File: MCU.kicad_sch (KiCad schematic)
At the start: 32 parts, among them J4 2125281600, J5 Conn_02x08_Odd_Even, J6 Conn_02x08_Odd_Even, U7 STM32F405RGTx, Y1 8MHz

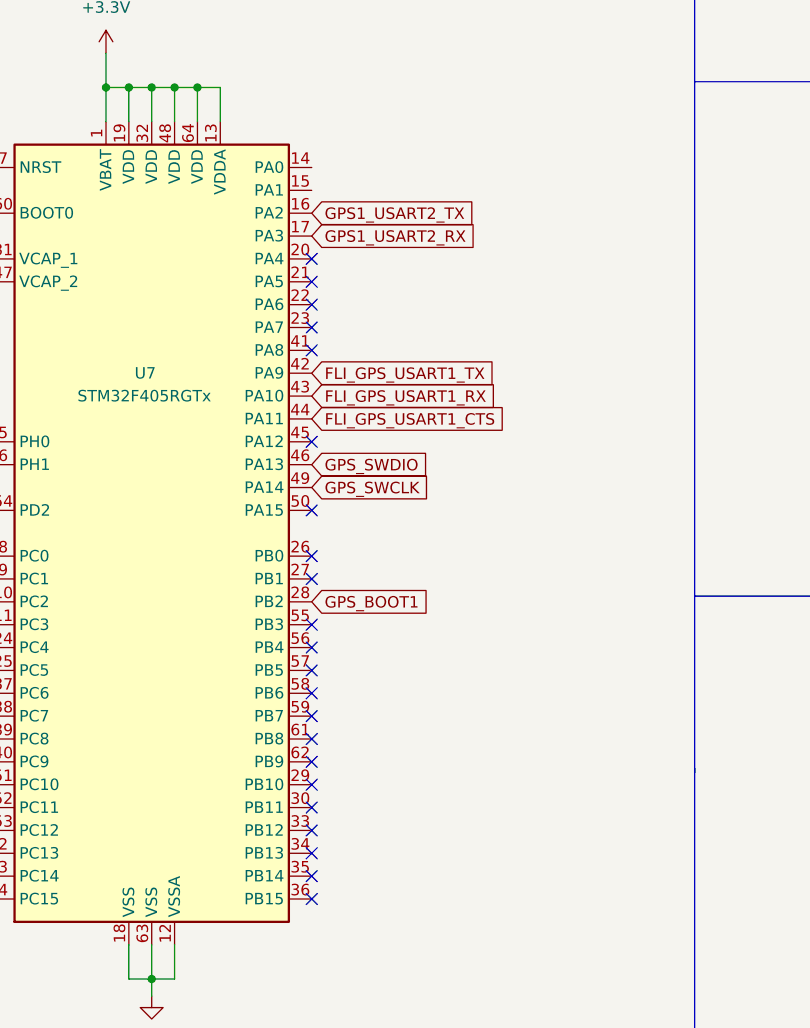
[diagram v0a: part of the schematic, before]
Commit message: Finished M10
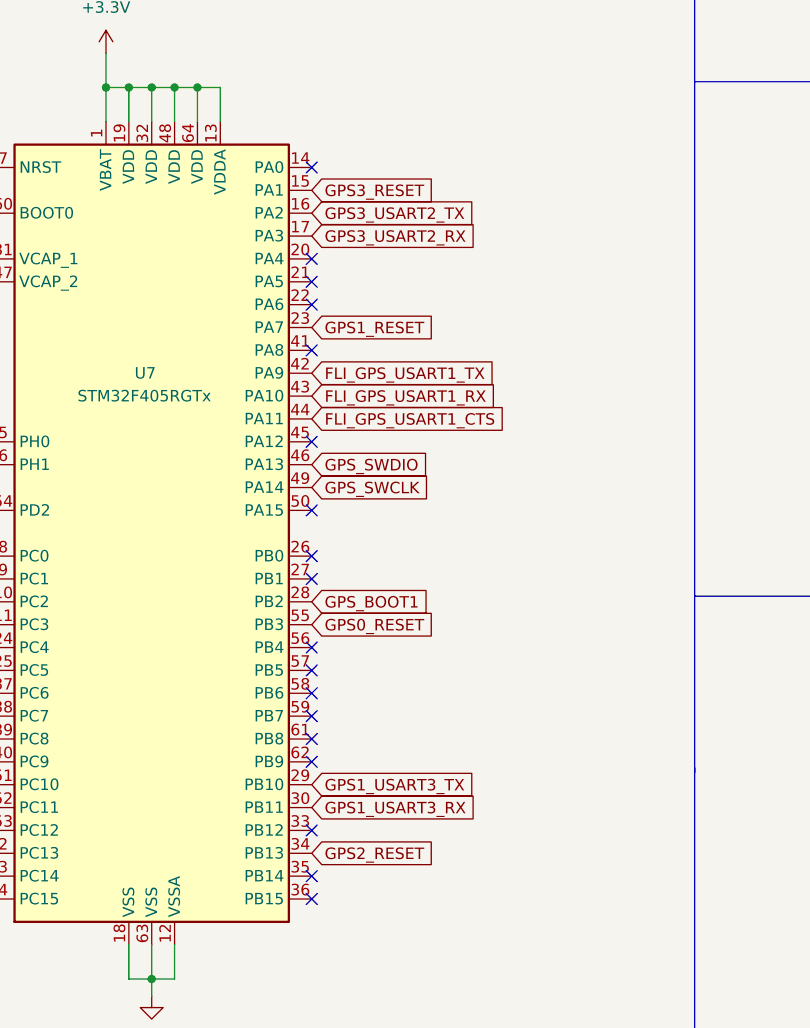
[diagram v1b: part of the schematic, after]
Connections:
- net GPS3_RESET: now reaches U7.15 (PA1)
- net GPS1_RESET: now reaches U7.23 (PA7)
- net GPS1_USART3_TX: now reaches U7.29 (PB10)
- net GPS1_USART3_RX: now reaches U7.30 (PB11)
- net GPS2_RESET: now reaches U7.34 (PB13)
- net GPS0_RESET: now reaches U7.55 (PB3)
- net GPS1_USART2_RX renamed GPS3_USART2_RX
- net GPS1_USART2_TX renamed GPS3_USART2_TX
- no-connect marks 40 -> 36
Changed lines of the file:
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@@
   (no_connect (at 139.7 127))
   (no_connect (at 219.71 97.79))
-  (no_connect (at 139.7 99.06))
   (no_connect (at 104.14 147.32))
   (no_connect (at 139.7 101.6))
@@
   (no_connect (at 139.7 137.16))
   (no_connect (at 139.7 119.38))
-  (no_connect (at 139.7 152.4))
   (no_connect (at 104.14 134.62))
   (no_connect (at 245.11 100.33))
@@
   (no_connect (at 245.11 97.79))
   (no_connect (at 104.14 132.08))
+  (no_connect (at 139.7 81.28))
   (no_connect (at 219.71 100.33))
   (no_connect (at 139.7 154.94))
   (no_connect (at 139.7 160.02))
   (no_connect (at 245.11 95.25))
-  (no_connect (at 139.7 149.86))
   (no_connect (at 139.7 96.52))
   (no_connect (at 104.14 137.16))
-  (no_connect (at 139.7 132.08))
-  (no_connect (at 139.7 157.48))
   (no_connect (at 104.14 144.78))
   (no_connect (at 104.14 124.46))
@@
     )
   )
+  (global_label "GPS2_RESET" (shape input) (at 139.7 157.48 0) (fields_autoplaced)
+    (effects (font (size 1.27 1.27)) (justify left))
+    (property "Intersheet References" "${INTERSHEET_REFS}" (id 0) (at 153.785 157.4006 0)
+      (effects (font (size 1.27 1.27)) (justify left) hide)
+    )
+  )
   (global_label "GPS_NRST" (shape input) (at 219.71 107.95 180) (fields_autoplaced)
     (effects (font (size 1.27 1.27)) (justify right))
@@
     )
   )
+  (global_label "GPS1_USART3_RX" (shape input) (at 139.7 152.4 0) (fields_autoplaced)
+    (effects (font (size 1.27 1.27)) (justify left))
+    (property "Intersheet References" "${INTERSHEET_REFS}" (id 0) (at 158.5626 152.3206 0)
+      (effects (font (size 1.27 1.27)) (justify left) hide)
+    )
+  )
   (global_label "GPS_BOOT1" (shape input) (at 40.005 44.45 180) (fields_autoplaced)
     (effects (font (size 1.27 1.27)) (justify right))
@@
     (property "Intersheet References" "${INTERSHEET_REFS}" (id 0) (at 198.4888 105.3306 0)
       (effects (font (size 1.27 1.27)) (justify right) hide)
+    )
+  )
+  (global_label "GPS3_RESET" (shape input) (at 139.7 83.82 0) (fields_autoplaced)
+    (effects (font (size 1.27 1.27)) (justify left))
+    (property "Intersheet References" "${INTERSHEET_REFS}" (id 0) (at 153.785 83.7406 0)
+      (effects (font (size 1.27 1.27)) (justify left) hide)
     )
   )
@@
     )
   )
-  (global_label "GPS1_USART2_TX" (shape input) (at 139.7 86.36 0) (fields_autoplaced)
+  (global_label "GPS3_USART2_TX" (shape input) (at 139.7 86.36 0) (fields_autoplaced)
     (effects (font (size 1.27 1.27)) (justify left))
     (property "Intersheet References" "${INTERSHEET_REFS}" (id 0) (at 158.2602 86.2806 0)
@@
     )
   )
+  (global_label "GPS1_RESET" (shape input) (at 139.7 99.06 0) (fields_autoplaced)
+    (effects (font (size 1.27 1.27)) (justify left))
+    (property "Intersheet References" "${INTERSHEET_REFS}" (id 0) (at 153.785 98.9806 0)
+      (effects (font (size 1.27 1.27)) (justify left) hide)
+    )
+  )
   (global_label "GPS_OSC_HSE_IN" (shape input) (at 60.325 199.39 0) (fields_autoplaced)
     (effects (font (size 1.27 1.27)) (justify left))
@@
     )
   )
+  (global_label "GPS1_USART3_TX" (shape input) (at 139.7 149.86 0) (fields_autoplaced)
+    (effects (font (size 1.27 1.27)) (justify left))
+    (property "Intersheet References" "${INTERSHEET_REFS}" (id 0) (at 158.2602 149.7806 0)
+      (effects (font (size 1.27 1.27)) (justify left) hide)
+    )
+  )
   (global_label "GPS_BOOT0" (shape input) (at 104.14 86.36 180) (fields_autoplaced)
     (effects (font (size 1.27 1.27)) (justify right))
@@
     )
   )
+  (global_label "GPS0_RESET" (shape input) (at 139.7 132.08 0) (fields_autoplaced)
+    (effects (font (size 1.27 1.27)) (justify left))
+    (property "Intersheet References" "${INTERSHEET_REFS}" (id 0) (at 153.785 132.0006 0)
+      (effects (font (size 1.27 1.27)) (justify left) hide)
+    )
+  )
   (global_label "GPS_DBG_UART4_TX" (shape input) (at 219.71 102.87 180) (fields_autoplaced)
     (effects (font (size 1.27 1.27)) (justify right))
@@
     )
   )
-  (global_label "GPS1_USART2_RX" (shape input) (at 139.7 88.9 0) (fields_autoplaced)
+  (global_label "GPS3_USART2_RX" (shape input) (at 139.7 88.9 0) (fields_autoplaced)
     (effects (font (size 1.27 1.27)) (justify left))
     (property "Intersheet References" "${INTERSHEET_REFS}" (id 0) (at 158.5626 88.8206 0)

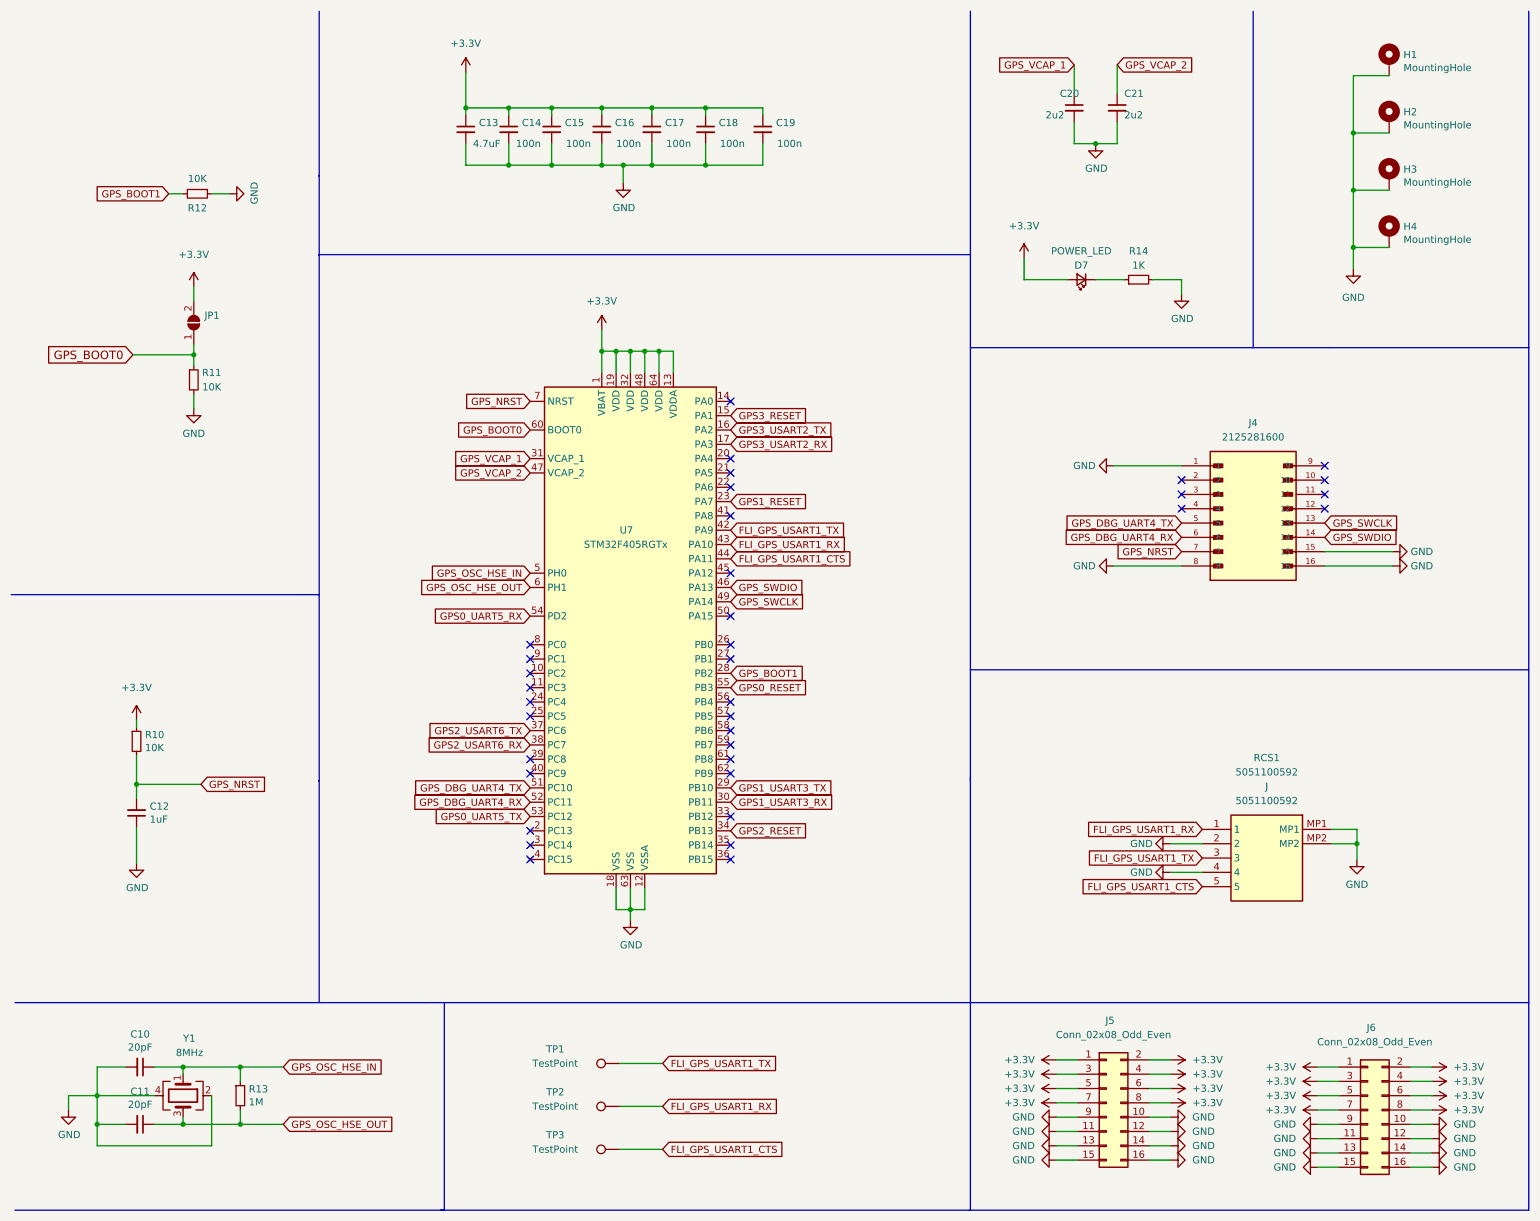
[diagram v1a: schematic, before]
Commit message: Last commit
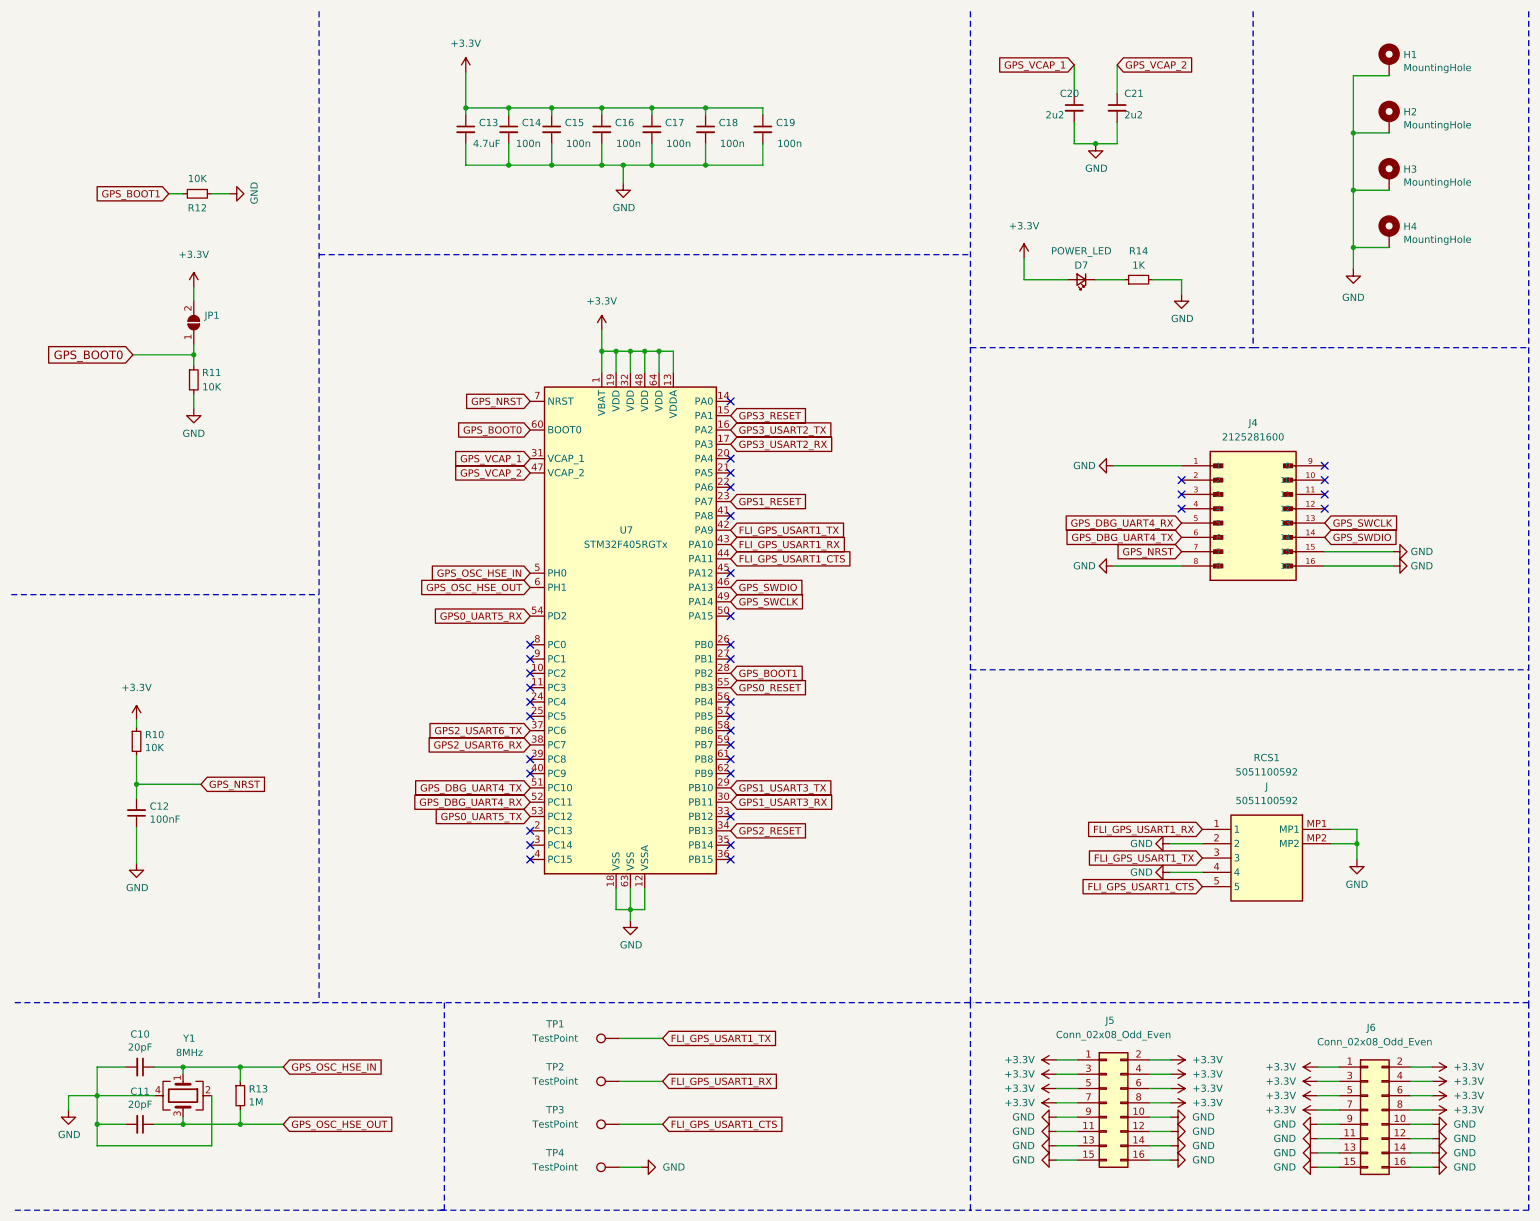
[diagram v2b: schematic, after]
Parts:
- added TP4: TestPoint, TestPoint:TestPoint_Pad_D1.0mm, symbol Connector:TestPoint
- C12: value 1uF -> 100nF
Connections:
- net GND: now also TP4.1
- net GPS_DBG_UART4_RX: now also J4.5; no longer J4.6
- net GPS_DBG_UART4_TX: now also J4.6; no longer J4.5
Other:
- moved on the sheet: TP1, TP2, TP3

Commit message: Second commit
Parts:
- removed JP1: SJumper, Jumper:SolderJumper-2_P1.3mm_Open_TrianglePad1.0x1.5mm, symbol Jumper:SolderJumper_2_Open
- added C28: 1uF, Capacitor_SMD:C_0402_1005Metric, symbol Device:C_Small
- added U5: SN74LV4052APWR, SN74LV4052APWR:PW16, symbol 2026-03-05_10-17-03:SN74LV4052APWR
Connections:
- net +3.3V: now also C28.1, U5.16 (VCC)
- net GND: now also C28.2, U5.7 (GND), U5.8 (GND)
- net GPS0_RESET: now also U7.57 (PB5); no longer U7.55 (PB3)
- net GPS0_UART5_RX: now also U5.12 (1Y0)
- net GPS0_UART5_TX: now also U5.1 (2Y0)
- net GPS1_RESET: now also U7.26 (PB0); no longer U7.23 (PA7)
- net GPS2_RESET: now also U7.39 (PC8); no longer U7.34 (PB13)
- net GPS2_USART6_RX: now also U5.11 (1Y3)
- net GPS2_USART6_TX: now also U5.4 (2Y3)
- net GPS_MUX_UART_RX: now reaches J4.10
- net GPS_MUX_UART_RX: now also U5.13 (1-COM)
- net GPS_MUX_UART_TX: now reaches J4.11
- net GPS_MUX_UART_TX: now also U5.3 (2-COM)
- net GPS_MUX_A: now reaches U7.59 (PB7)
- net GPS_MUX_A: now also U5.10 (A)
- net GPS_MUX_B: now reaches U7.61 (PB8)
- net GPS_MUX_B: now also U5.9 (B)
- net GPS_MUX_INH: now reaches U7.62 (PB9)
- net GPS_MUX_INH: now also U5.6 (INH)
- net GPS1_USART3_RX: no longer names the net of U7.30 (PB11)
- net GPS1_USART3_TX: no longer names the net of U7.29 (PB10)
- net GPS3_RESET: no longer names the net of U7.15 (PA1)
- net GPS3_USART2_RX renamed GPS1_USART2_RX
- net GPS1_USART2_RX: now also U5.14 (1Y1)
- net GPS3_USART2_TX renamed GPS1_USART2_TX
- net GPS1_USART2_TX: now also U5.5 (2Y1)
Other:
- moved on the sheet: C10, C11, C12, C13, C14, C15, C16, C17, C18, C19, C20, C21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
